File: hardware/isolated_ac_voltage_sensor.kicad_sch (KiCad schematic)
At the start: 18 parts, among them U2 MCP4161-xxxx-P, U3 LM358

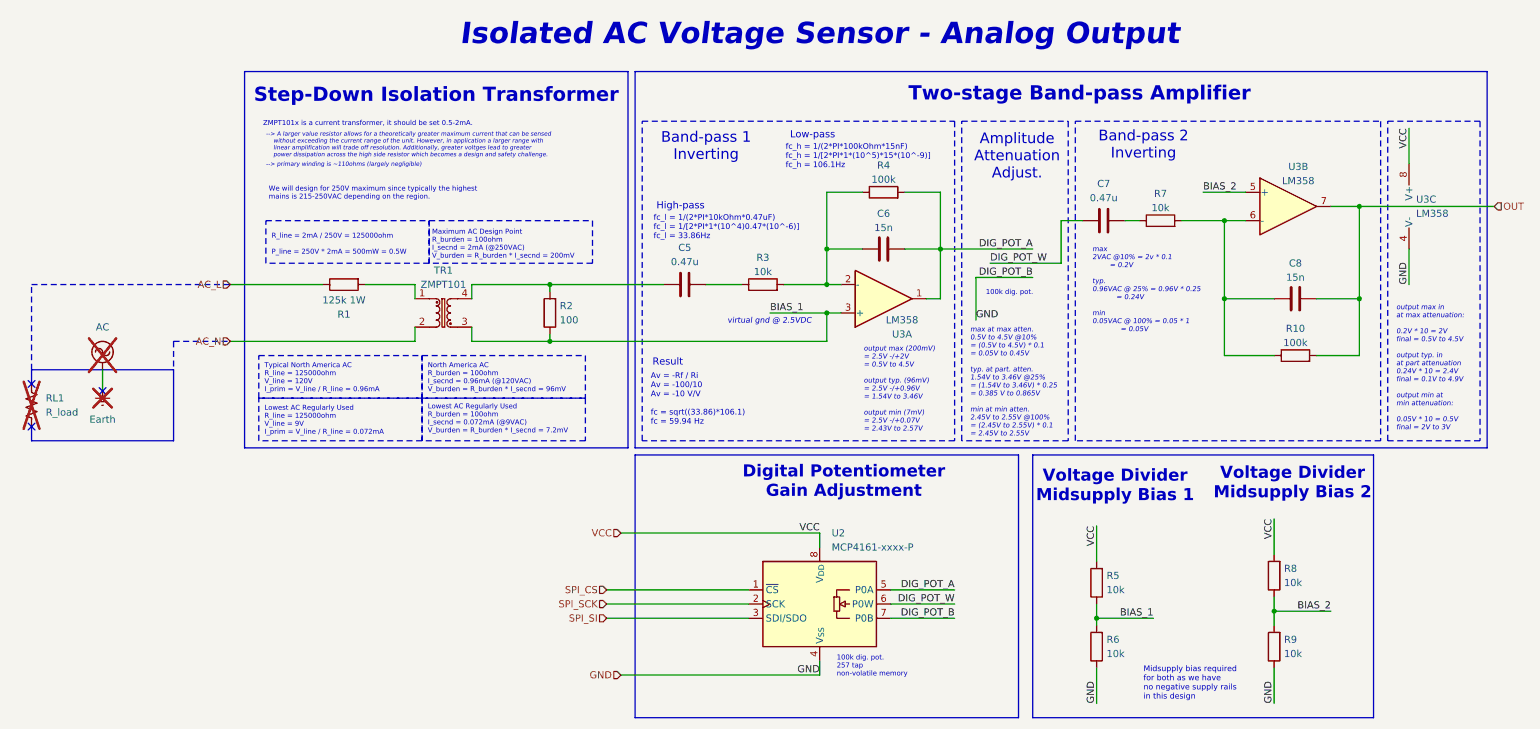
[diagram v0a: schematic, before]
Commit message: finalized pcb
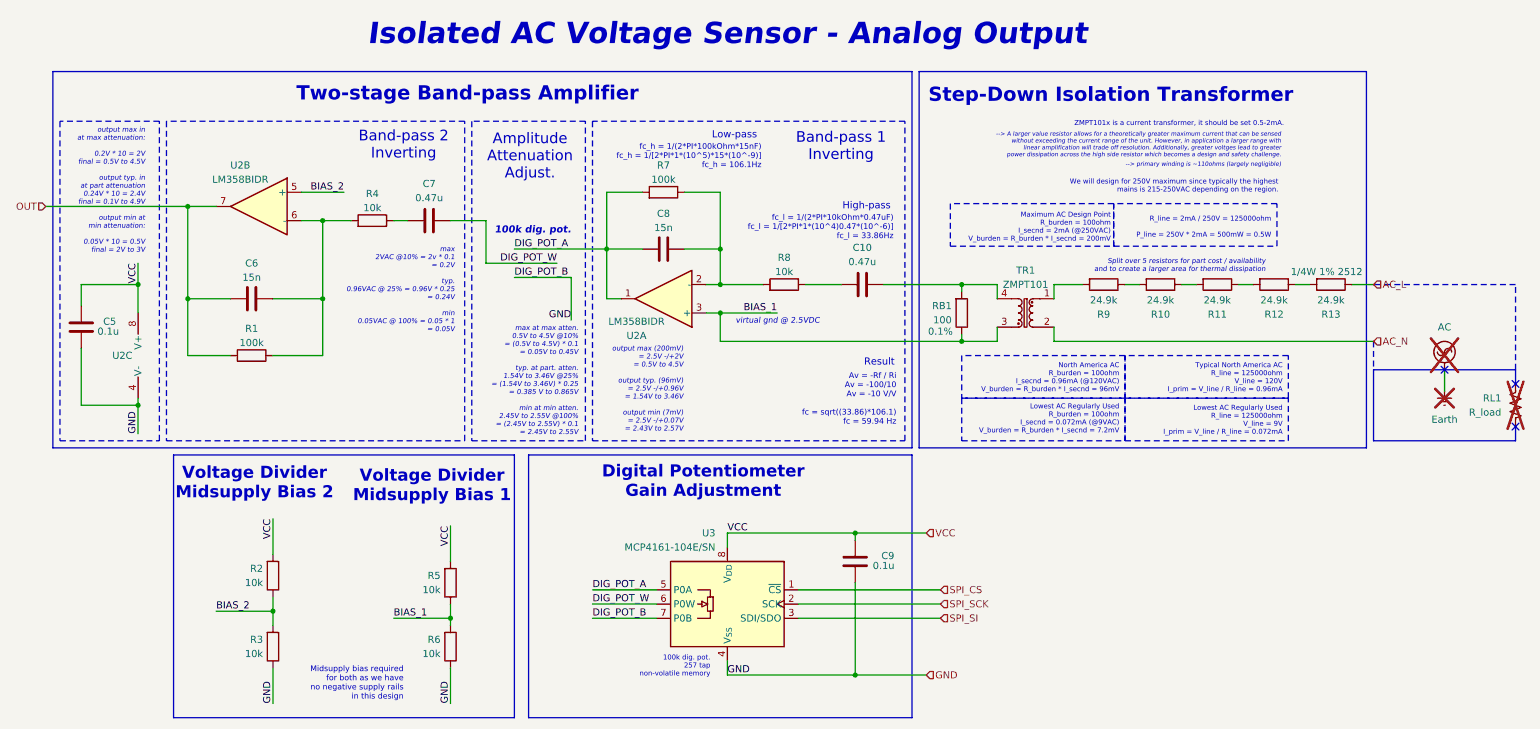
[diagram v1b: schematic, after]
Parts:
- added C5, C9: 0.1u, Capacitor_SMD:C_0805_2012Metric_Pad1.18x1.45mm_HandSolder, symbol Device:C
- added R10, R11, R12, R9: 24.9k, Resistor_SMD:R_1206_3216Metric_Pad1.30x1.75mm_HandSolder, symbol Device:R
- C10: renamed from C5; footprint (none) -> Capacitor_SMD:C_0805_2012Metric_Pad1.18x1.45mm_HandSolder
- C6: renamed from C8; footprint (none) -> Capacitor_SMD:C_0805_2012Metric_Pad1.18x1.45mm_HandSolder
- C7: footprint (none) -> Capacitor_SMD:C_0805_2012Metric_Pad1.18x1.45mm_HandSolder
- C8: renamed from C6; footprint (none) -> Capacitor_SMD:C_0805_2012Metric_Pad1.18x1.45mm_HandSolder
- R1: renamed from R10; footprint (none) -> Resistor_SMD:R_0805_2012Metric_Pad1.20x1.40mm_HandSolder
- R13: renamed from R1; value 125k 1W -> 24.9k; footprint (none) -> Resistor_SMD:R_1206_3216Metric_Pad1.30x1.75mm_HandSolder; Specs (none) -> 1/4W 1% 2512
- R2: renamed from R8; footprint (none) -> Resistor_SMD:R_0805_2012Metric_Pad1.20x1.40mm_HandSolder
- R3: renamed from R9; footprint (none) -> Resistor_SMD:R_0805_2012Metric_Pad1.20x1.40mm_HandSolder
- R4: renamed from R7; footprint (none) -> Resistor_SMD:R_0805_2012Metric_Pad1.20x1.40mm_HandSolder
- R5, R6: footprint (none) -> Resistor_SMD:R_0805_2012Metric_Pad1.20x1.40mm_HandSolder
- R7: renamed from R4; footprint (none) -> Resistor_SMD:R_0805_2012Metric_Pad1.20x1.40mm_HandSolder
- R8: renamed from R3; footprint (none) -> Resistor_SMD:R_0805_2012Metric_Pad1.20x1.40mm_HandSolder
- RB1: renamed from R2; footprint (none) -> Resistor_SMD:R_0805_2012Metric_Pad1.20x1.40mm_HandSolder; Specs (none) -> 0.1%
- U2: renamed from U3; value LM358 -> LM358BIDR; footprint (none) -> Package_SO:SOIC-8_3.9x4.9mm_P1.27mm
- U3: renamed from U2; value MCP4161-xxxx-P -> MCP4161-104E/SN; footprint Package_DIP:DIP-8_W7.62mm -> Package_SO:SOIC-8_3.9x4.9mm_P1.27mm
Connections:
- net GND: now also C5.1, C9.1
- net VCC: now also C5.2, C9.2
- net at R13.2: now also R12.1; no longer TR1.1
- new net: R11.1, R12.2
- new net: R10.2, R9.1
- new net: R9.2, TR1.1
- new net: R10.1, R11.2
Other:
- note added: "Split over 5 resistors for part cost / availability and to create a larger area for thermal dissipation"
- moved on the sheet: C10, C6, C7, C8, R1, R13, R2, R3, R4, R5, R6, R7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
